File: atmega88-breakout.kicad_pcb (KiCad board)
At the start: 2 copper layers, 46.7 x 15.2 mm, 12 parts, among them J1 Conn_01x08_Male, J2 ICSP Header, J4 Conn_01x08_Male, U1 ATmega88PA-AU

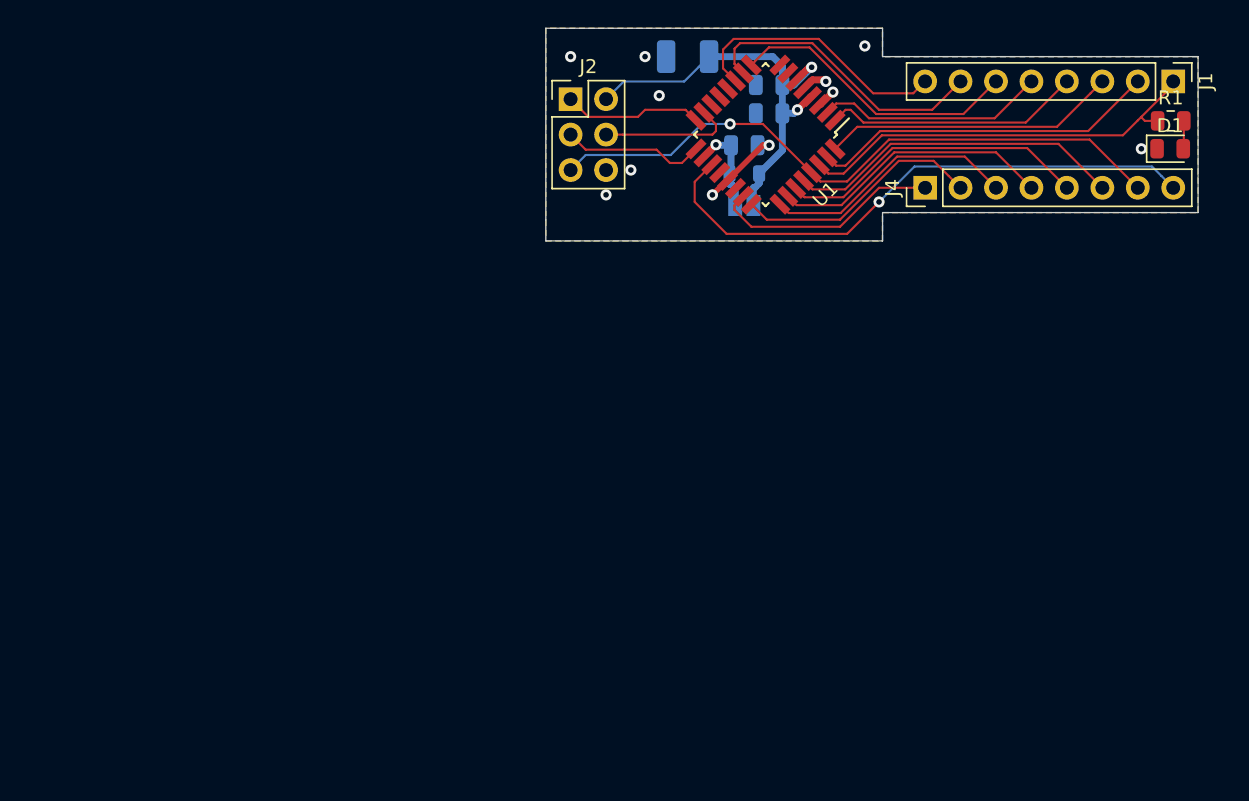
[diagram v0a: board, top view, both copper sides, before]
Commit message: Rev A release (ordered)
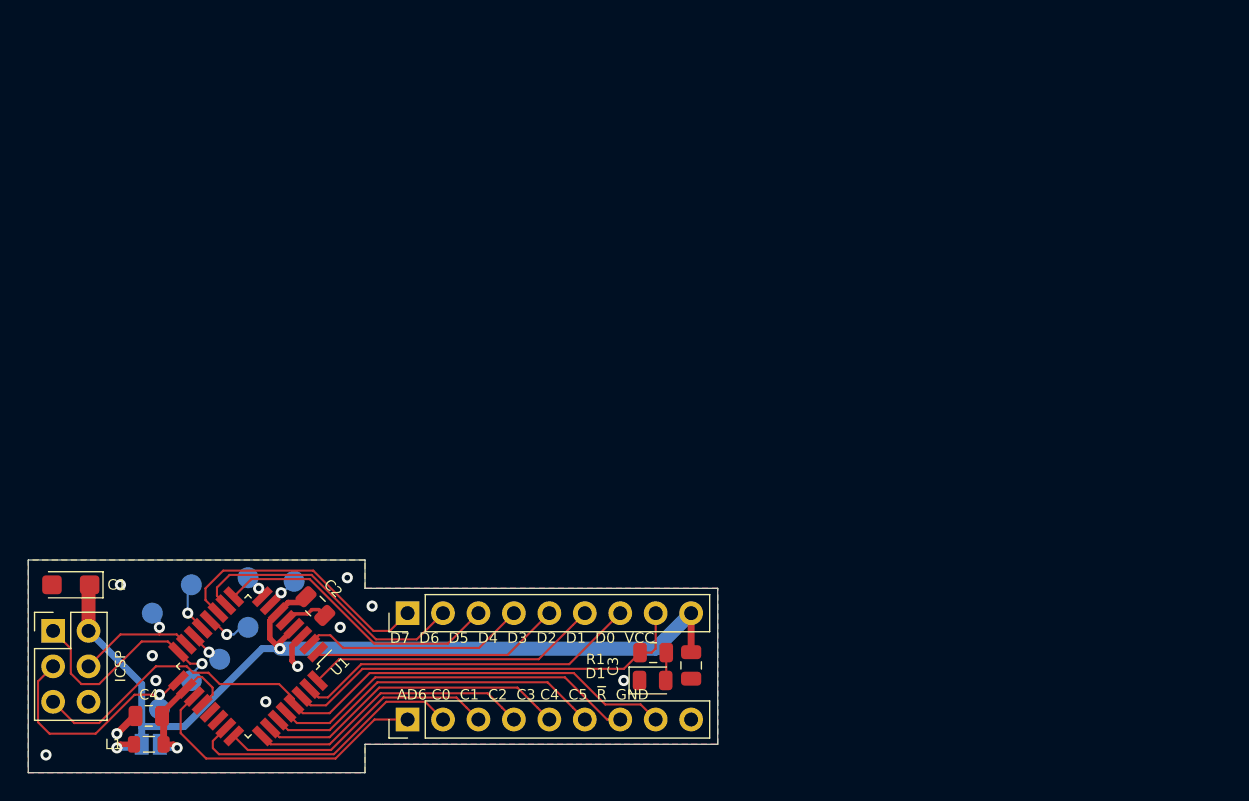
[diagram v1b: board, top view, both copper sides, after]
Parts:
- removed J4: Conn_01x08_Male, Connector_PinHeader_2.54mm:PinHeader_1x08_P2.54mm_Vertical
- added B0: TestPoint, TestPoint:TestPoint_Pad_D1.5mm, B.Cu at (134.4, 102.6)
- added B1: TestPoint, TestPoint:TestPoint_Pad_D1.5mm, B.Cu at (130.3, 99.6)
- added B2: TestPoint, TestPoint:TestPoint_Pad_D1.5mm, B.Cu at (132.3, 104.9)
- added B3: TestPoint, TestPoint:TestPoint_Pad_D1.5mm, B.Cu at (127.5, 101.6)
- added B4: TestPoint, TestPoint:TestPoint_Pad_D1.5mm, B.Cu at (130.3, 106.4)
- added B5: TestPoint, TestPoint:TestPoint_Pad_D1.5mm, B.Cu at (128.0, 108.5)
- added B6: TestPoint, TestPoint:TestPoint_Pad_D1.5mm, B.Cu at (137.7, 99.3)
- added B7: TestPoint, TestPoint:TestPoint_Pad_D1.5mm, B.Cu at (134.4, 99.1)
- added J3: Conn_01x09, Connector_PinHeader_2.54mm:PinHeader_1x09_P2.54mm_Vertical, F.Cu at (145.8, 101.6)
- C1: footprint Capacitor_Tantalum_SMD:CP_EIA-3528-12_Kemet-T -> Capacitor_Tantalum_SMD:CP_EIA-3216-18_Kemet-A; moved to F.Cu
- C2, C3, C4, L1: moved to F.Cu
- J1: value Conn_01x08_Male -> Conn_01x09; footprint Connector_PinHeader_2.54mm:PinHeader_1x08_P2.54mm_Vertical -> Connector_PinHeader_2.54mm:PinHeader_1x09_P2.54mm_Vertical
- R1: value R_Small -> 1k
- moved J1 71.4 mm to (145.8, 109.2), turned to 90 degrees
- moved L1 59.1 mm to (127.3, 111.0), turned to 0 degrees
- moved C4 59.1 mm to (127.3, 109.0), turned to 0 degrees
- moved C1 58.2 mm to (121.7, 99.6)
- moved JP1 57.4 mm to (127.4, 111.0), turned to 0 degrees
- moved D1 53.2 mm to (163.4, 106.4)
- moved ICSP 53.2 mm to (120.4, 102.9)
- moved R1 53.2 mm to (163.4, 104.4)
- moved U1 53.2 mm to (134.4, 105.4)
- moved C2 49.5 mm to (139.2, 101.1), turned to 135 degrees
- moved C3 40.0 mm to (166.1, 105.3), turned to 90 degrees
- renumbered J2 to ICSP
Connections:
- J1 pad 1: /D0 -> ADC6
- J1 pad 2: /D1 -> /C0
- J1 pad 3: /D2 -> /C1
- J1 pad 4: /D3 -> /C2
- J1 pad 5: /D4 -> /C3
- J1 pad 6: /D5 -> /C4
- J1 pad 7: /D6 -> /C5
- J1 pad 8: /D7 -> /C6
- U1 pad 12: (no net) -> /B0
- U1 pad 13: (no net) -> /B1
- U1 pad 14: (no net) -> /B2
- U1 pad 20: (no net) -> VAA
- U1 pad 22: (no net) -> ADC7
- U1 pad 7: (no net) -> /B6
- U1 pad 8: (no net) -> /B7
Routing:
- net VCC: track 31.8 -> 70.2 mm
- net ADC6: track 41.0 -> 21.2 mm, vias 1 -> 0
- net /B5: track 10.2 -> 17.4 mm, vias 0 -> 1
- net /B4: track 10.0 -> 16.7 mm, vias 0 -> 1
- net VAA: track 6.93 -> 11.3 mm
- net /C0: track 16.6 -> 20.6 mm
- net /B1: track 0.00 -> 3.65 mm, vias 0 -> 1
- net /B0: track 0.00 -> 3.35 mm, vias 0 -> 1
- net /C6: track 46.4 -> 49.7 mm, vias 1 -> 0
- net /B2: track 0.00 -> 2.55 mm, vias 0 -> 1
- net /C5: track 24.3 -> 26.9 mm
- net /C4: track 22.3 -> 24.8 mm
- net /B6: track 0.00 -> 2.45 mm, vias 0 -> 1
- net /C3: track 20.3 -> 22.7 mm
- net /C2: track 18.4 -> 20.6 mm
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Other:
- board size 46.7 x 15.2 mm -> 49.4 x 15.2 mm
- board text added: "AD6 C0 C1 C2 C3 C4 C5 ~R~ GND"
- board text added: "D7 D6 D5 D4 D3 D2 D1 D0 VCC"
